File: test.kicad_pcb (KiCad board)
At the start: 2 copper layers, 47 x 92.7 mm, 6 parts, among them J1 Conn_01x32_Female, J2 Conn_01x32_Female, J3 DB9_Male, J4 Conn_01x32_Female, J5 Conn_01x32_Female, U1 MCP2551-I-SN

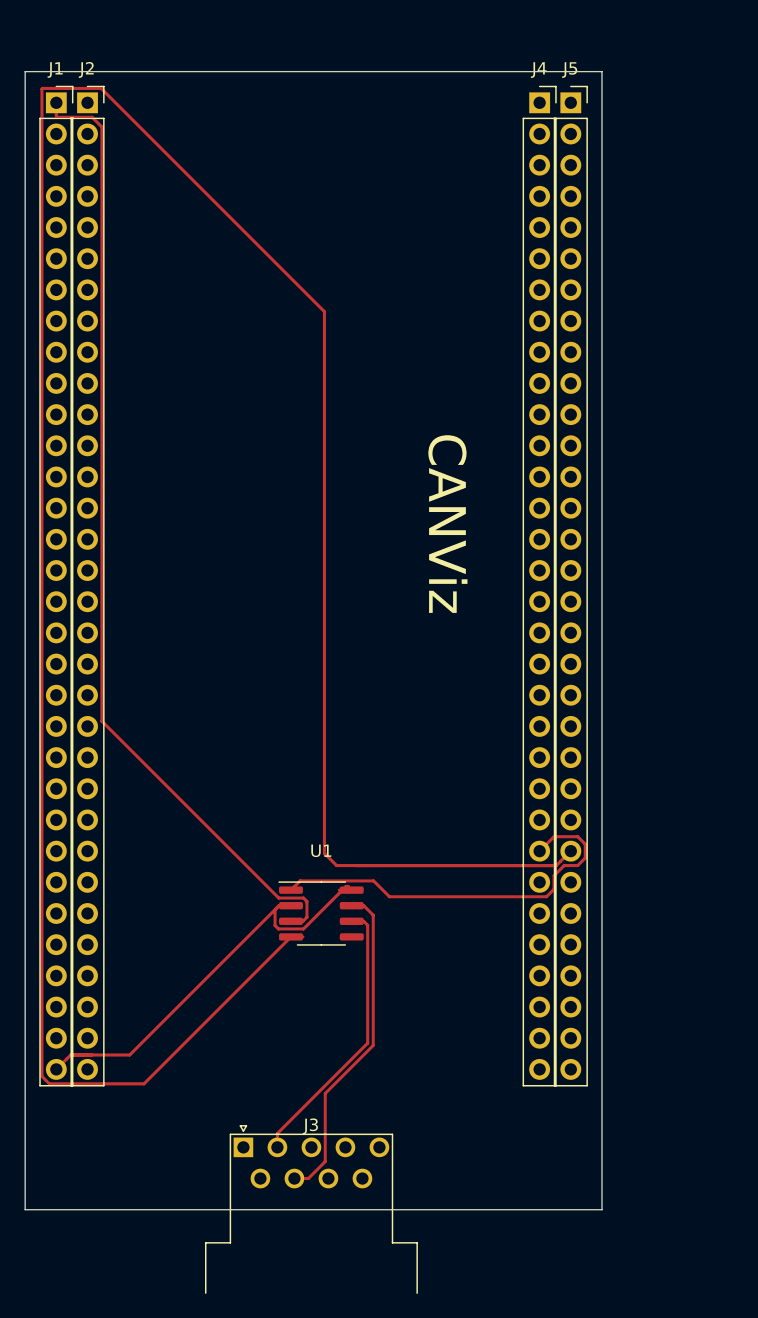
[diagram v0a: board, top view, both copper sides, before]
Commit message: Update db9 position for CAD
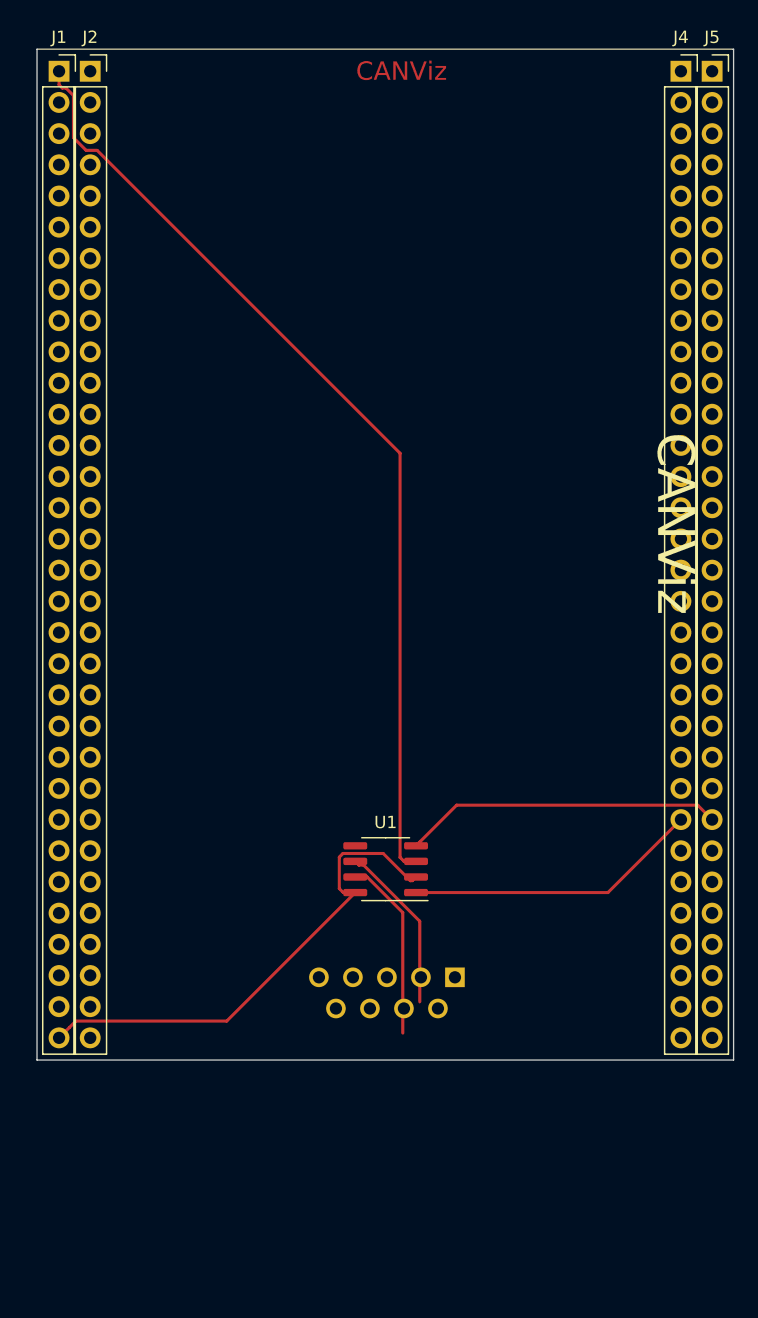
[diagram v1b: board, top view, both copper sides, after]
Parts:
- J3: moved to B.Cu
- moved J3 22.1 mm to (88.3, 136.0), turned to 180 degrees
- moved J4 11.8 mm to (106.8, 62.2)
- moved J5 11.8 mm to (109.3, 62.2)
- moved U1 6.36 mm to (82.7, 127.2), turned to 180 degrees
- moved J1 2.58 mm to (56.1, 62.2)
- moved J2 2.58 mm to (58.6, 62.2)
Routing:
- net PB12: track 218.9 -> 26.0 mm
- net canH: track 26.8 -> 14.9 mm
- net canL: track 22.6 -> 13.8 mm
- net PB13: track 32.3 -> 24.0 mm
- net GND_STM: track 37.1 -> 40.4 mm
- net +5V_STM: track 79.1 -> 77.7 mm
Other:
- board size 47 x 92.7 mm -> 56.7 x 82.3 mm
